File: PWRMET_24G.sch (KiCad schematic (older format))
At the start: 0 parts

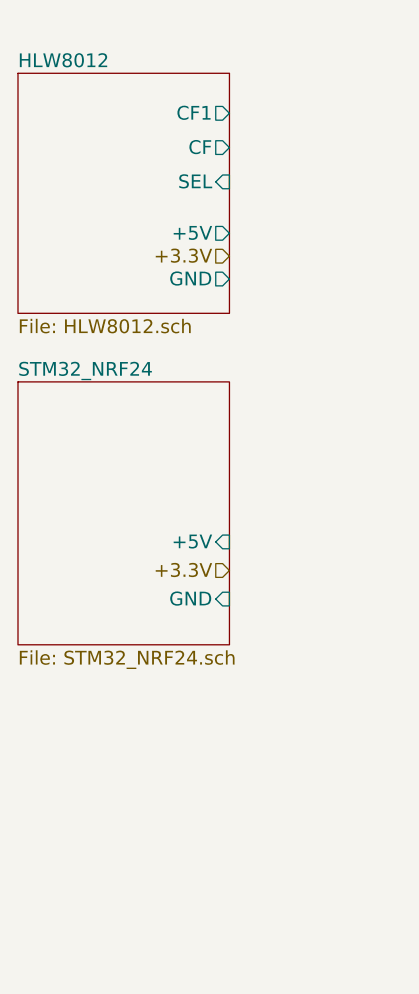
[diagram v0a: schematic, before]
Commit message: upd
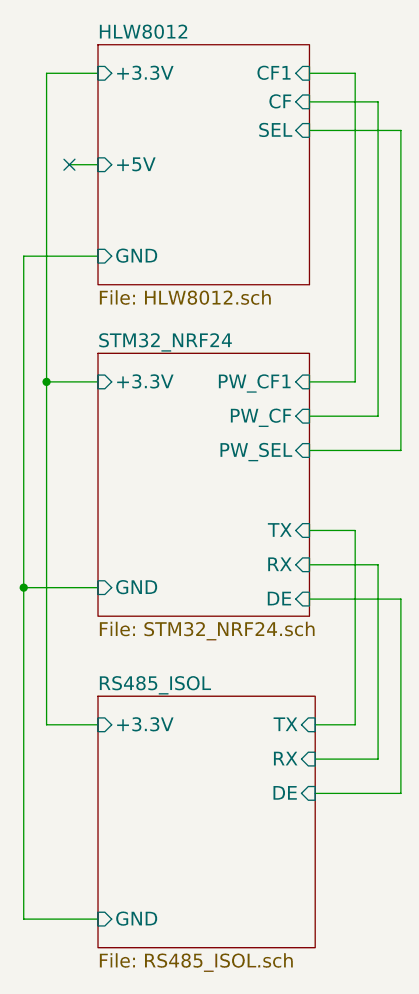
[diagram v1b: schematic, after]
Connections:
- no-connect marks 0 -> 1
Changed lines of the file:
@@
 LIBS:contrib
 LIBS:valves
+LIBS:stm32
+LIBS:BK_Common
+LIBS:BK_LED_Drivers
 LIBS:BK_STM8
-LIBS:BK_Common
-LIBS:stm32
 LIBS:PWRMET_24G-cache
 EELAYER 25 0
@@
 $Descr A4 11693 8268
 encoding utf-8
-Sheet 1 3
+Sheet 1 4
 Title ""
 Date ""
@@
 $EndDescr
 $Sheet
-S 1775 2025 925  1050
+S 2125 3250 925  1150
+U 591CC0DB
+F0 "STM32_NRF24" 60
+F1 "STM32_NRF24.sch" 60
+F2 "PW_CF" I R 3050 3525 60
+F3 "PW_CF1" I R 3050 3375 60
+F4 "TX" I R 3050 4025 60
+F5 "RX" I R 3050 4175 60
+F6 "PW_SEL" I R 3050 3675 60
+F7 "DE" I R 3050 4325 60
+F8 "+3.3V" I L 2125 3375 60
+F9 "GND" I L 2125 4275 60
+$EndSheet
+$Sheet
+S 2125 1900 925  1050
 U 591C108A
 F0 "HLW8012" 60
 F1 "HLW8012.sch" 60
-F2 "CF" O R 2700 2350 60
-F3 "CF1" O R 2700 2200 60
-F4 "SEL" I R 2700 2500 60
-F5 "+5V" O R 2700 2725 60
-F6 "GND" O R 2700 2925 60
+F2 "+3.3V" I L 2125 2025 60
+F3 "+5V" I L 2125 2425 60
+F4 "GND" I L 2125 2825 60
+F5 "CF1" I R 3050 2025 60
+F6 "CF" I R 3050 2150 60
+F7 "SEL" I R 3050 2275 60
 $EndSheet
+Wire Wire Line
+	3050 3375 3250 3375
+Wire Wire Line
+	3250 3375 3250 2025
+Wire Wire Line
+	3250 2025 3050 2025
+Wire Wire Line
+	3050 3525 3350 3525
+Wire Wire Line
+	3350 3525 3350 2150
+Wire Wire Line
+	3350 2150 3050 2150
+Wire Wire Line
+	3050 3675 3450 3675
+Wire Wire Line
+	3450 3675 3450 2275
+Wire Wire Line
+	3450 2275 3050 2275
+Wire Wire Line
+	2125 2825 1800 2825
+Wire Wire Line
+	1800 2825 1800 5725
+Wire Wire Line
+	1800 4275 2125 4275
+Wire Wire Line
+	2125 3375 1900 3375
+Wire Wire Line
+	1900 2025 1900 4875
+Wire Wire Line
+	1900 2025 2125 2025
 $Sheet
-S 1775 3375 925  1150
-U 591CC0DB
-F0 "STM32_NRF24" 60
-F1 "STM32_NRF24.sch" 60
-F2 "GND" I R 2700 4325 60
-F3 "+5V" I R 2700 4075 60
+S 2125 4750 950  1100
+U 59219A27
+F0 "RS485_ISOL" 60
+F1 "RS485_ISOL.sch" 60
+F2 "GND" I L 2125 5725 60
+F3 "+3.3V" I L 2125 4875 60
+F4 "RX" I R 3075 5025 60
+F5 "TX" I R 3075 4875 60
+F6 "DE" I R 3075 5175 60
 $EndSheet
-Text HLabel 2700 2825 0    60   Input ~ 0
-+3.3V
-Text HLabel 2700 4200 0    60   Input ~ 0
-+3.3V
+Wire Wire Line
+	1900 4875 2125 4875
+Connection ~ 1900 3375
+Wire Wire Line
+	1800 5725 2125 5725
+Connection ~ 1800 4275
+Wire Wire Line
+	3075 4875 3250 4875
+Wire Wire Line
+	3250 4875 3250 4025
+Wire Wire Line
+	3250 4025 3050 4025
+Wire Wire Line
+	3075 5025 3350 5025
+Wire Wire Line
+	3350 5025 3350 4175
+Wire Wire Line
+	3350 4175 3050 4175
+Wire Wire Line
+	3075 5175 3450 5175
+Wire Wire Line
+	3450 5175 3450 4325
+Wire Wire Line
+	3450 4325 3050 4325
+Wire Wire Line
+	2125 2425 2000 2425
+NoConn ~ 2000 2425
 $EndSCHEMATC
